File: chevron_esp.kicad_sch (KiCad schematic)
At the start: 20 parts, among them J1 282837-4, K1 SRD-05VDC-SL-C, K2 SRD-05VDC-SL-C, K3 SRD-05VDC-SL-C, P1 282837-2, Q1 PN2222A, Q2 PN2222A, Q3 PN2222A, SW1 1825057-2, U1 ESP32-DEVKIT-V1, U2 RA-02_LORA

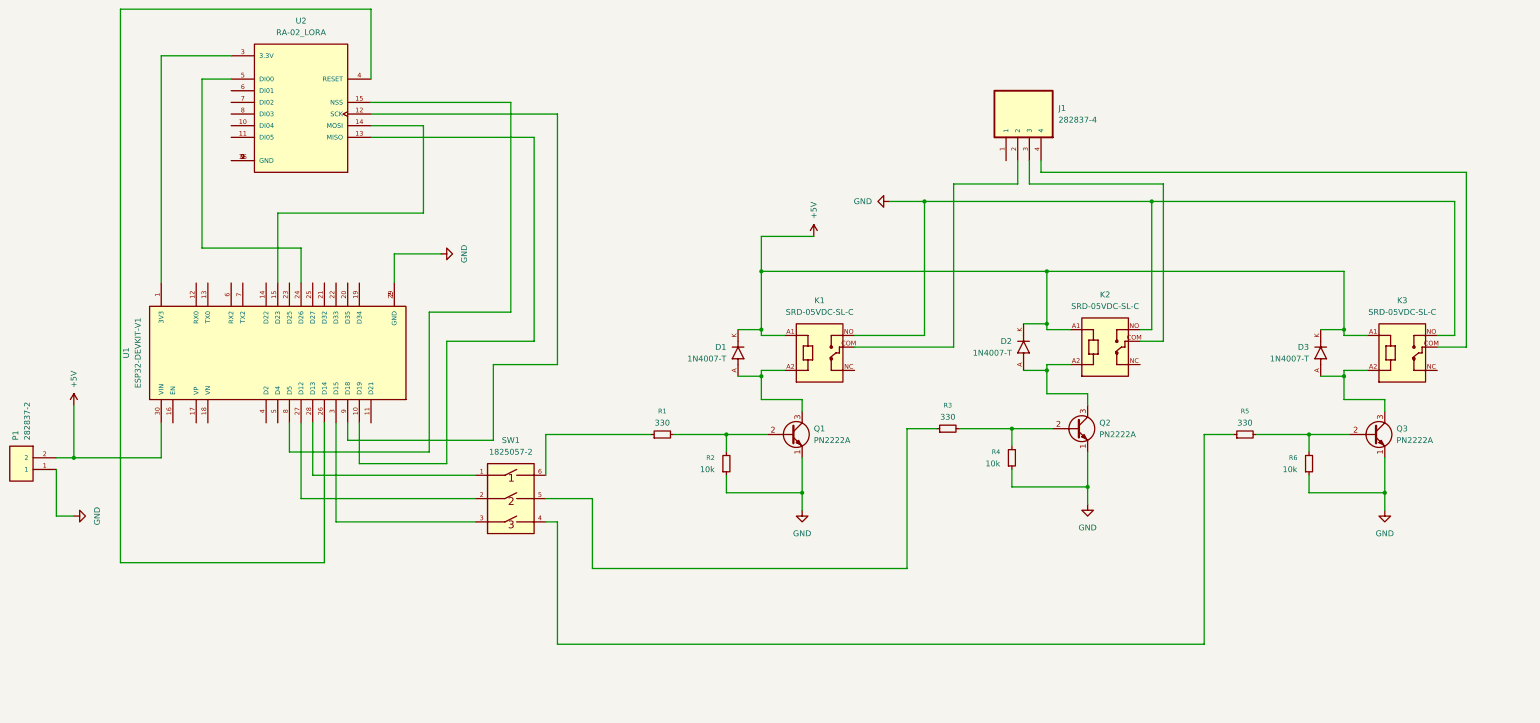
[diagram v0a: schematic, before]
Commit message: chevron esp v1.2
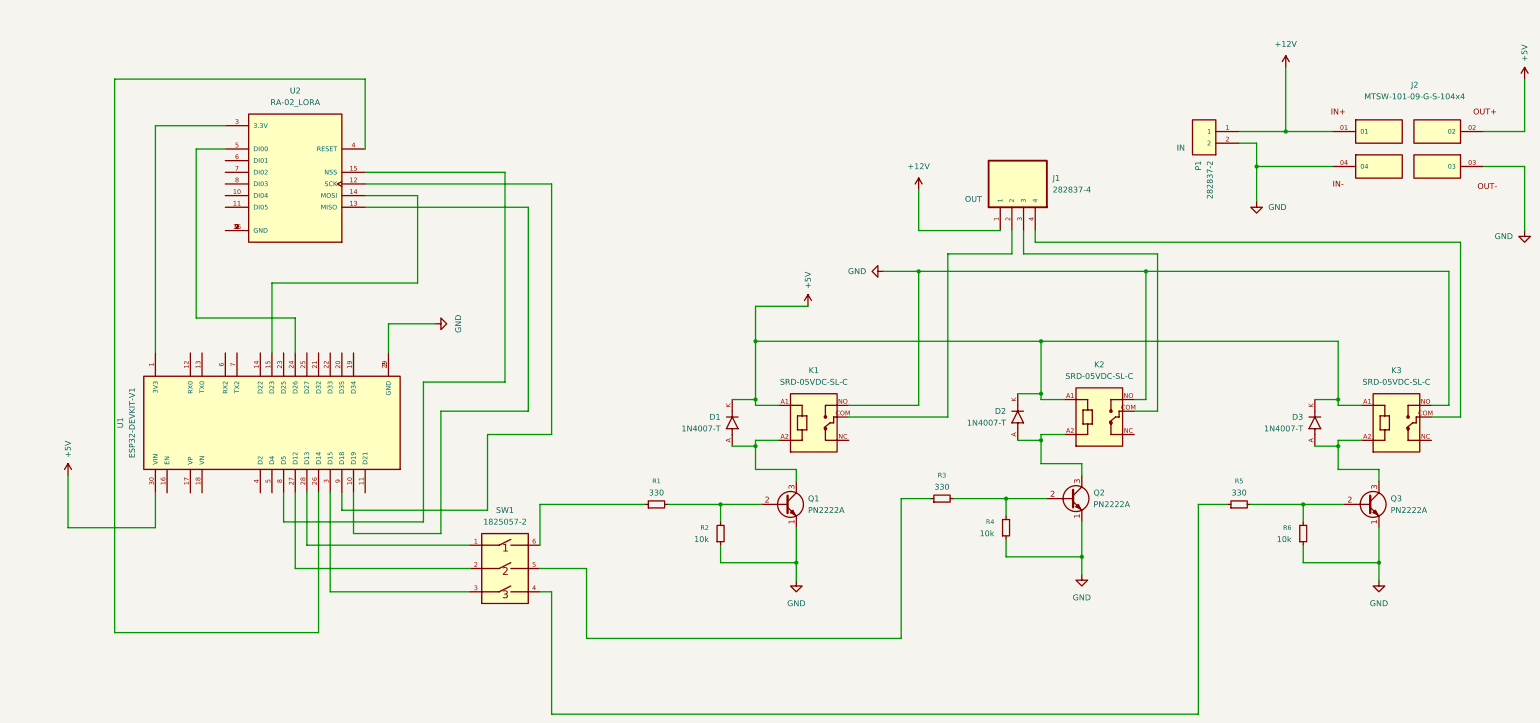
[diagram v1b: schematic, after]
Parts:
- added J2: MTSW-101-09-G-S-104x4, MTSW-101-09-G-S-104:SAMTEC_MTSW-101-09-G-S-104x4, symbol MTSW-101-09-G-S-104:MTSW-101-09-G-S-104x4
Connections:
- net +5V: now also J2.02; no longer P1.2
- net GND: now also P1.2, J2.03, J2.04; no longer P1.1
- net +12V: now reaches J1.1
- net +12V: now also P1.1, J2.01
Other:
- note added: "IN"
- note added: "OUT"
- moved on the sheet: D1, D2, D3, J1, K1, K2, K3, P1, Q1, Q2, Q3, R1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
